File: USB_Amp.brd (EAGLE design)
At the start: 87 x 60 mm, 192 parts, among them CON1 AUDIO_IN, CON2 PROG, CON3 PWR IN, CON4 USB-C-2OZ, CON5 SWD, IC1 ISO7762, IC10 74LVC1G79, IC11 1.8V, IC12 AK1110, IC13 STM32G030F, IC14 CH221, IC15 7808, IC16 TAR5SB33, IC2 3.3V, IC3 PIC32MZEF, IC4 TAR5SB33, IC5 SSM3582, IC6 3G04, IC7 TL431, IC8 74LVC1G79, IC9 74LVC1G79, Q1 PNP, Q2 PNP, Q3 PNP, Q4 NPN, Q5 NPN, X1 12MHz, X2 22.5792MHz, X3 24.576MHz

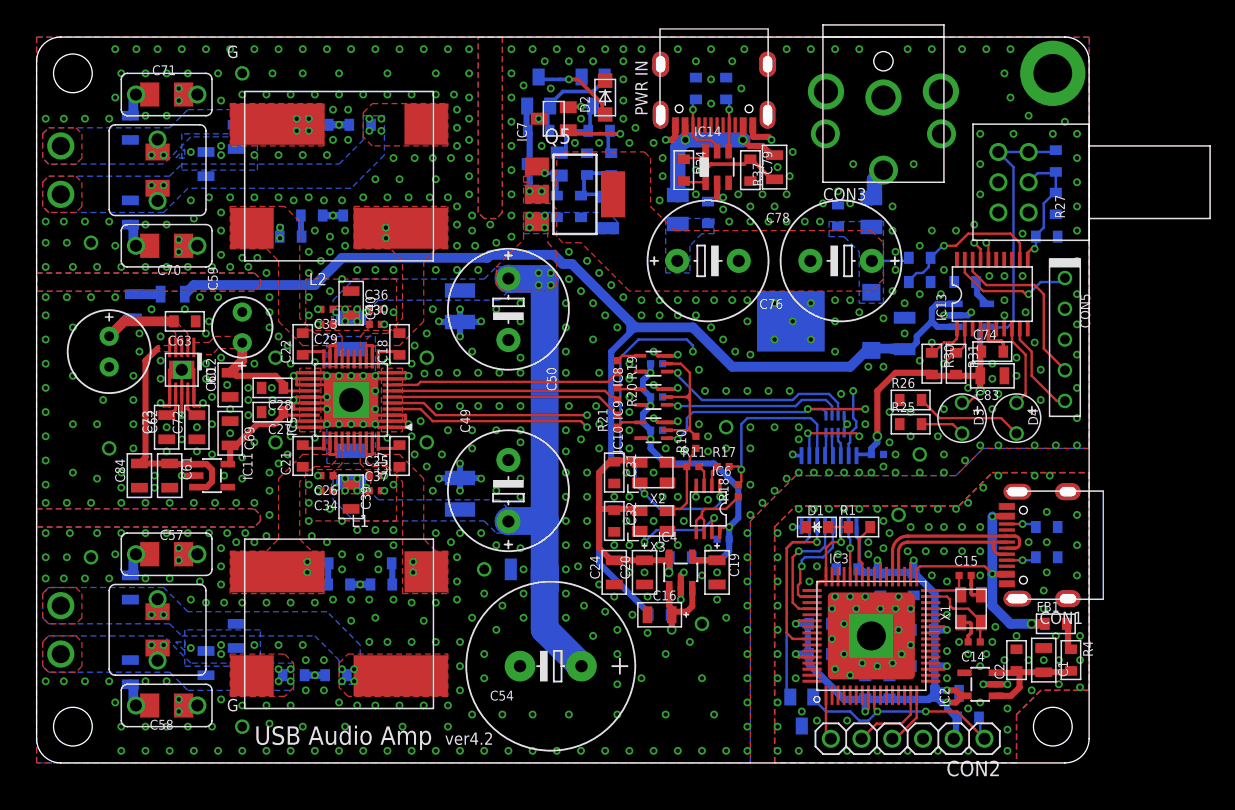
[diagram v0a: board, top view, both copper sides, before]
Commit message: 微修正
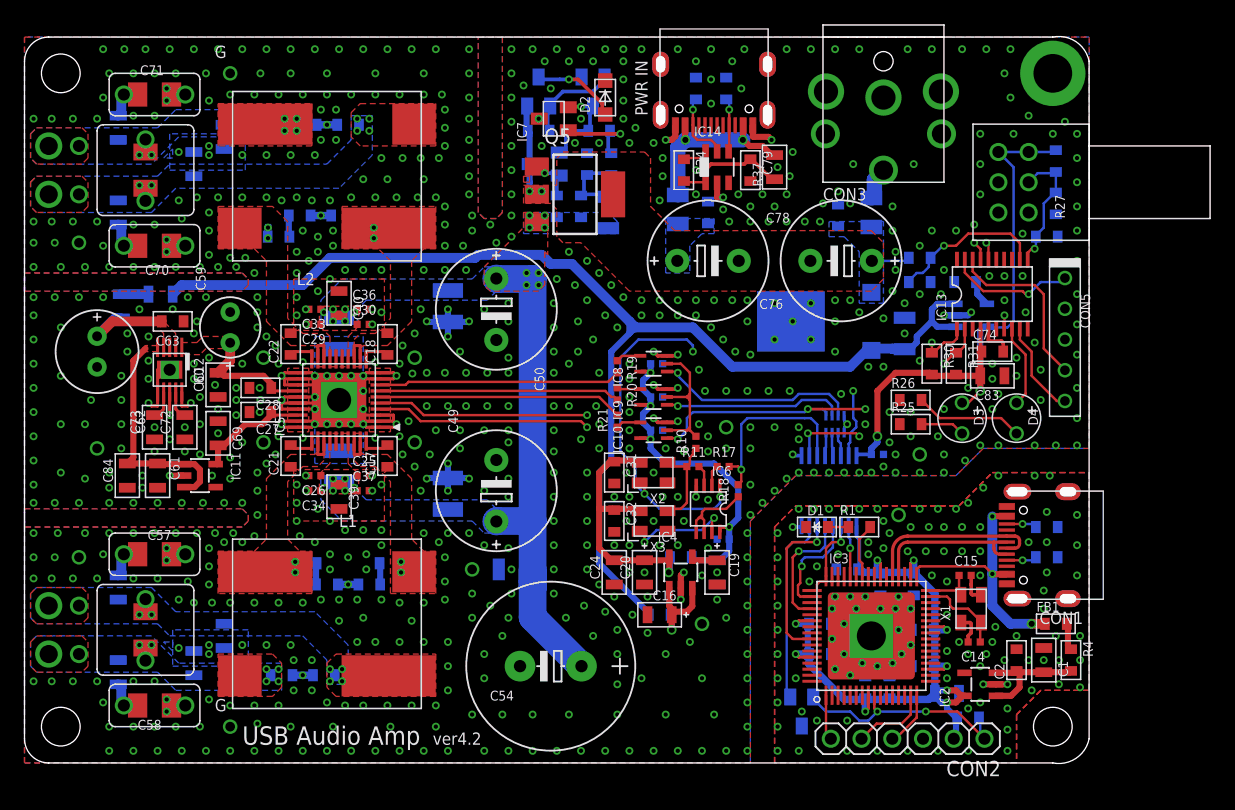
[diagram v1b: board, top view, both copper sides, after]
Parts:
- added TP19, TP20: L_P, my_connector:TESTPIN-MID
- added TP21, TP22: R_N, my_connector:TESTPIN-MID
- L1, L2: value 7uH -> 7uH-UA8013
- R20: value LRCLK -> DATA
- R21: value DATA -> LRCLK
- moved C17 1.00 mm to (29.0, 25.4)
- moved C18 1.00 mm to (29.0, 34.6)
- moved C21 1.00 mm to (21.0, 25.4)
- moved C22 1.00 mm to (21.0, 34.6)
- moved C25 1.00 mm to (27.0, 23.8)
- moved C26 1.00 mm to (23.0, 23.8)
- moved C27 1.00 mm to (18.5, 29.0)
- moved C28 1.00 mm to (18.5, 31.0)
- moved C29 1.00 mm to (23.0, 36.2)
- moved C30 1.00 mm to (27.0, 36.2)
- moved C33 1.00 mm to (23.0, 37.5)
- moved C34 1.00 mm to (23.0, 22.5)
- moved C36 1.00 mm to (27.0, 37.5)
- moved C37 1.00 mm to (27.0, 22.5)
- moved C39 1.00 mm to (25.0, 22.0)
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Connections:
- net SPK_OUTN_L: now also TP19.1
- net SPK_OUTN_R: now also TP22.1
- net SPK_OUTP_L: now also TP20.1
- net SPK_OUTP_R: now also TP21.1
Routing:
- net GND: track 103.3 -> 98.6 mm, vias 773 -> 777
- net I2S_SCK_BUF: track 19.0 -> 20.0 mm
- net I2S_LRCLK_BUF: track 19.2 -> 20.2 mm
- net I2S_DATA_BUF: track 18.9 -> 19.9 mm
- net I2C_SDA: track 56.8 -> 57.8 mm
- net I2C_SCL: track 60.2 -> 61.2 mm
- net +8V: track 101.8 -> 102.8 mm
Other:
- board size 87 x 60 mm -> 88 x 60.1 mm
